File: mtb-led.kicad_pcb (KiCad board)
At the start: 2 copper layers, 120 x 50 mm, 57 parts, among them J7 AVR-ISP-6, J9 DEBUG, SW1 SW_Push, U1 ATmega328PB-A, U2 78M05, U3 TLC5940PWP, U4 TLC5940PWP, U5 MAX487E, Y1 14.7456 MHz

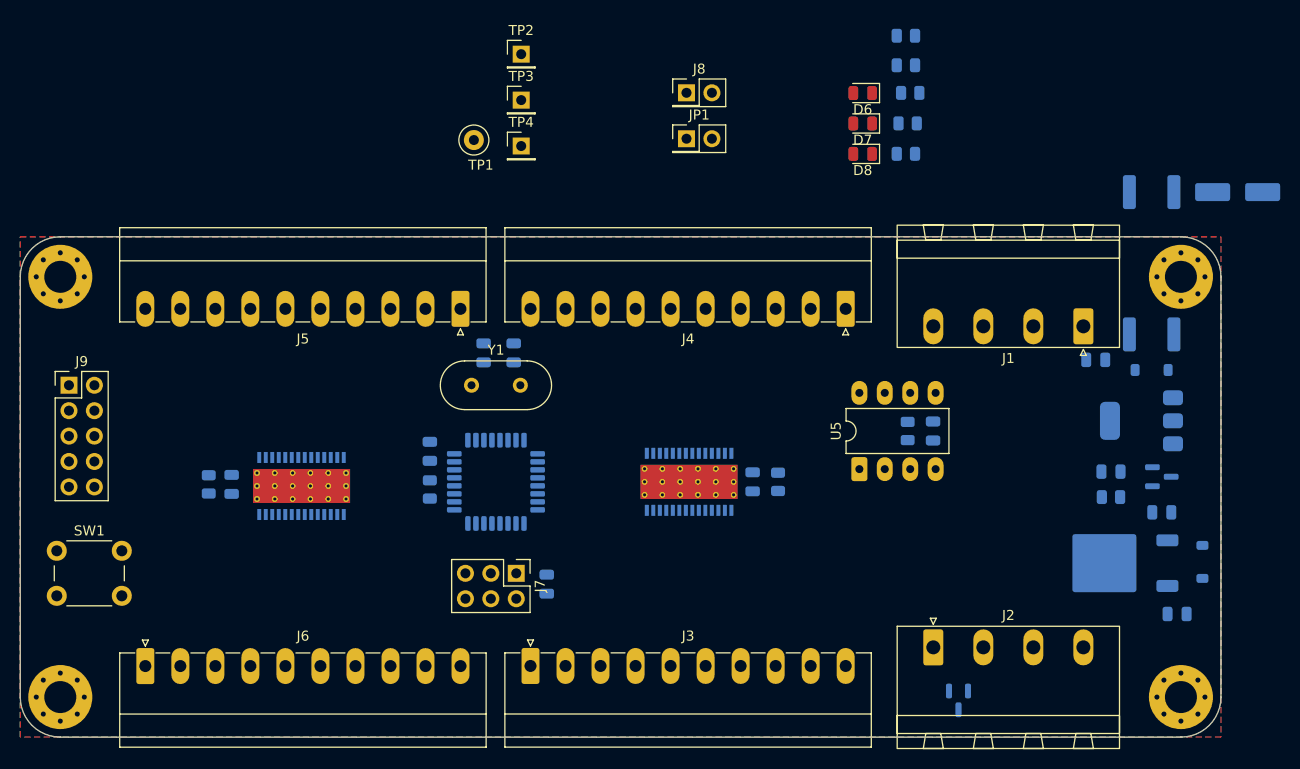
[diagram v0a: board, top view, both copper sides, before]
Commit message: PCB: wire, wire, ...
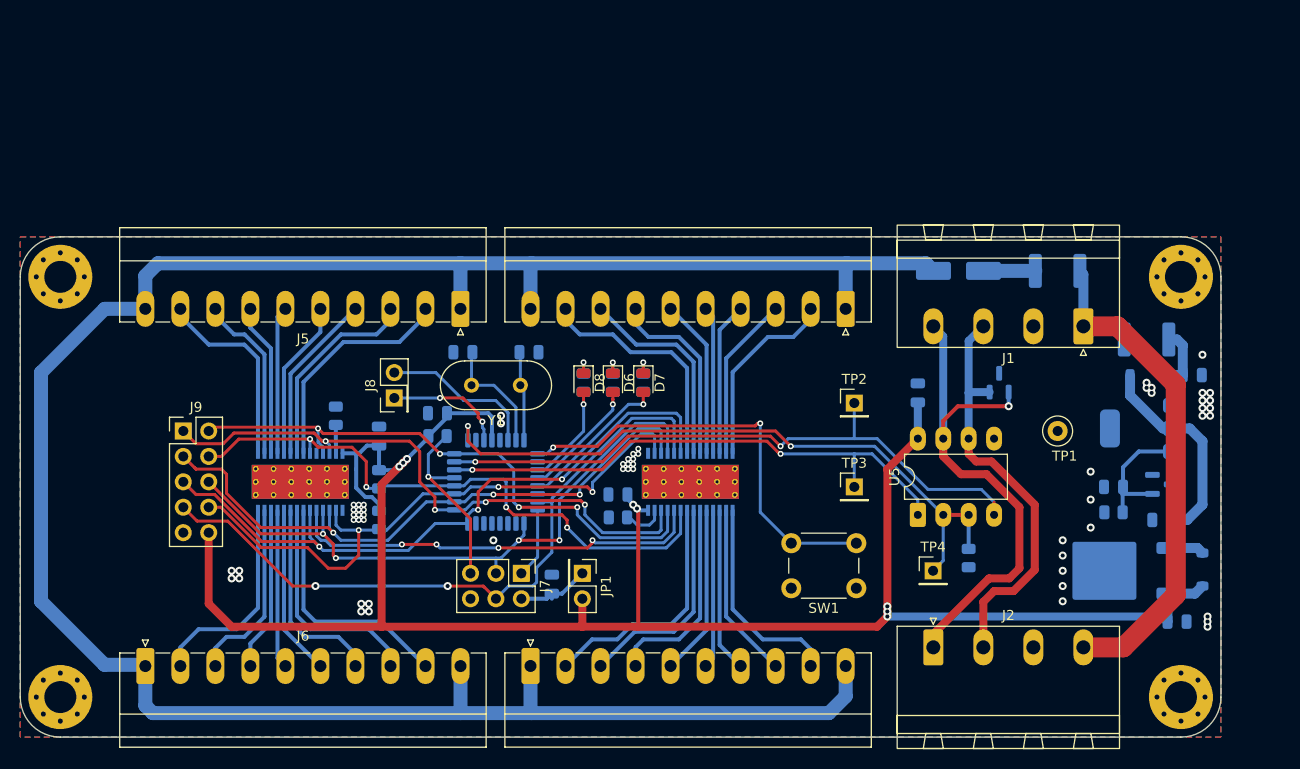
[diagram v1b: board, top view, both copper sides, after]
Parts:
- moved SW1 80.0 mm to (165.6, 105.1), turned to 180 degrees
- moved R10 71.5 mm to (117.9, 98.3), turned to -90 degrees
- moved R9 67.0 mm to (117.9, 94.2), turned to -90 degrees
- moved TP1 65.2 mm to (185.7, 89.4)
- moved TP4 59.1 mm to (173.2, 103.4)
- moved TP3 51.0 mm to (165.4, 95.0)
- moved TP2 48.2 mm to (165.4, 86.6)
- moved JP1 44.7 mm to (138.2, 103.6), turned to -90 degrees
- moved J8 42.2 mm to (119.4, 86.1), turned to 90 degrees
- moved R7 41.5 mm to (141.2, 84.6), turned to 90 degrees
- moved R6 39.5 mm to (138.3, 84.6), turned to 90 degrees
- moved D6 38.2 mm to (141.2, 84.6), turned to -90 degrees
- moved R8 37.0 mm to (144.3, 84.6), turned to 90 degrees
- moved D8 36.1 mm to (138.3, 84.6), turned to -90 degrees
- moved D7 33.9 mm to (144.3, 84.6), turned to -90 degrees
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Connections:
- net Net-(U1-PD5) renamed /BTN
- J3 pad 2: /OUT7 -> /OUT15
- J3 pad 3: /OUT6 -> /OUT14
- J3 pad 4: /OUT5 -> /OUT13
- J3 pad 5: /OUT4 -> /OUT12
- J3 pad 6: /OUT3 -> /OUT11
- J3 pad 7: /OUT2 -> /OUT10
- J3 pad 8: /OUT1 -> /OUT9
- J3 pad 9: /OUT0 -> /OUT8
- J4 pad 2: /OUT15 -> /OUT7
- J4 pad 3: /OUT14 -> /OUT6
- J4 pad 4: /OUT13 -> /OUT5
- J4 pad 5: /OUT12 -> /OUT4
- J4 pad 6: /OUT11 -> /OUT3
- J4 pad 7: /OUT10 -> /OUT2
- J4 pad 8: /OUT9 -> /OUT1
- J4 pad 9: /OUT8 -> /OUT0
- J5 pad 2: /OUT23 -> /OUT31
- J5 pad 3: /OUT22 -> /OUT30
- J5 pad 4: /OUT21 -> /OUT29
- J5 pad 5: /OUT20 -> /OUT28
- J5 pad 6: /OUT19 -> /OUT27
- J5 pad 7: /OUT18 -> /OUT26
- J5 pad 8: /OUT17 -> /OUT25
- J5 pad 9: /OUT16 -> /OUT24
- J6 pad 2: /OUT31 -> /OUT23
- J6 pad 3: /OUT30 -> /OUT22
- J6 pad 4: /OUT29 -> /OUT21
- J6 pad 5: /OUT28 -> /OUT20
- J6 pad 6: /OUT27 -> /OUT19
- J6 pad 7: /OUT26 -> /OUT18
- J6 pad 8: /OUT25 -> /OUT17
- J6 pad 9: /OUT24 -> /OUT16
- J9 pad 1: /VPRG -> /DCPRG
- J9 pad 2: /XLAT -> /GSCLK
- J9 pad 3: /DCPRG -> /XLAT
- J9 pad 5: /GSCLK -> /VPRG
- J9 pad 7: /BLANK -> /MOSI
- J9 pad 8: /MOSI -> /BLANK
- U1 pad 11: unconnected-(U1-PD7-Pad11) -> /LED_RED
- U1 pad 23: /LED_RED -> unconnected-(U1-PC0-Pad23)
- U1 pad 26: /BLANK -> /XLAT
- U1 pad 27: /XLAT -> /BLANK
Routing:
- net +12V: track 0.00 -> 233.1 mm
- net +5V: track 0.00 -> 200.2 mm, vias 0 -> 8
- net /MOSI: track 0.00 -> 69.1 mm, vias 0 -> 2
- net /VPRG: track 0.00 -> 67.5 mm, vias 0 -> 3
- net /MTB-DE: track 0.00 -> 67.3 mm, vias 0 -> 2
- net /SCK: track 0.00 -> 66.2 mm, vias 0 -> 4
- net /MTB-TX: track 0.00 -> 63.2 mm, vias 0 -> 2
- net /XLAT: track 0.00 -> 62.3 mm, vias 0 -> 3
- net /BLANK: track 0.00 -> 60.9 mm, vias 0 -> 3
- net /XERR: track 0.00 -> 60.9 mm, vias 0 -> 4
- net /DCPRG: track 0.00 -> 60.2 mm, vias 0 -> 4
- net /GSCLK: track 0.00 -> 58.0 mm, vias 0 -> 4
- net /MTB-RX: track 0.00 -> 54.8 mm, vias 0 -> 2
- net /+12V-IN: track 0.00 -> 54.4 mm
- net /BUS-: track 0.00 -> 52.2 mm, vias 0 -> 1
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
